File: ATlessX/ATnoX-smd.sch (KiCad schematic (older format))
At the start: 32 parts, among them J1 EXT_PWR_SW, J2 ATX, J3 AT, J4 PWR_LED, SW1 Power, U1 74LS74, U2 74LS14, U3 L7905

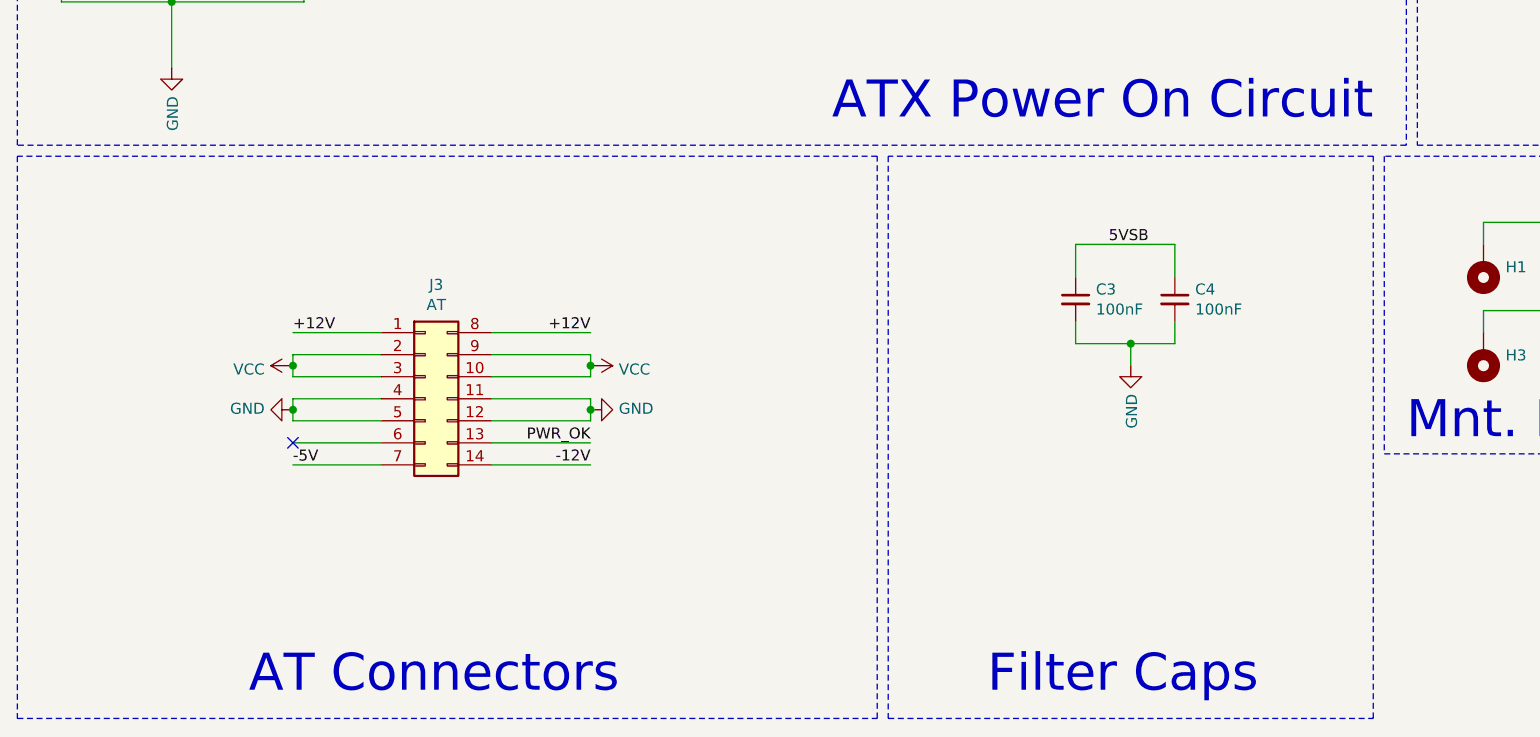
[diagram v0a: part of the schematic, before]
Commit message: Rev 3
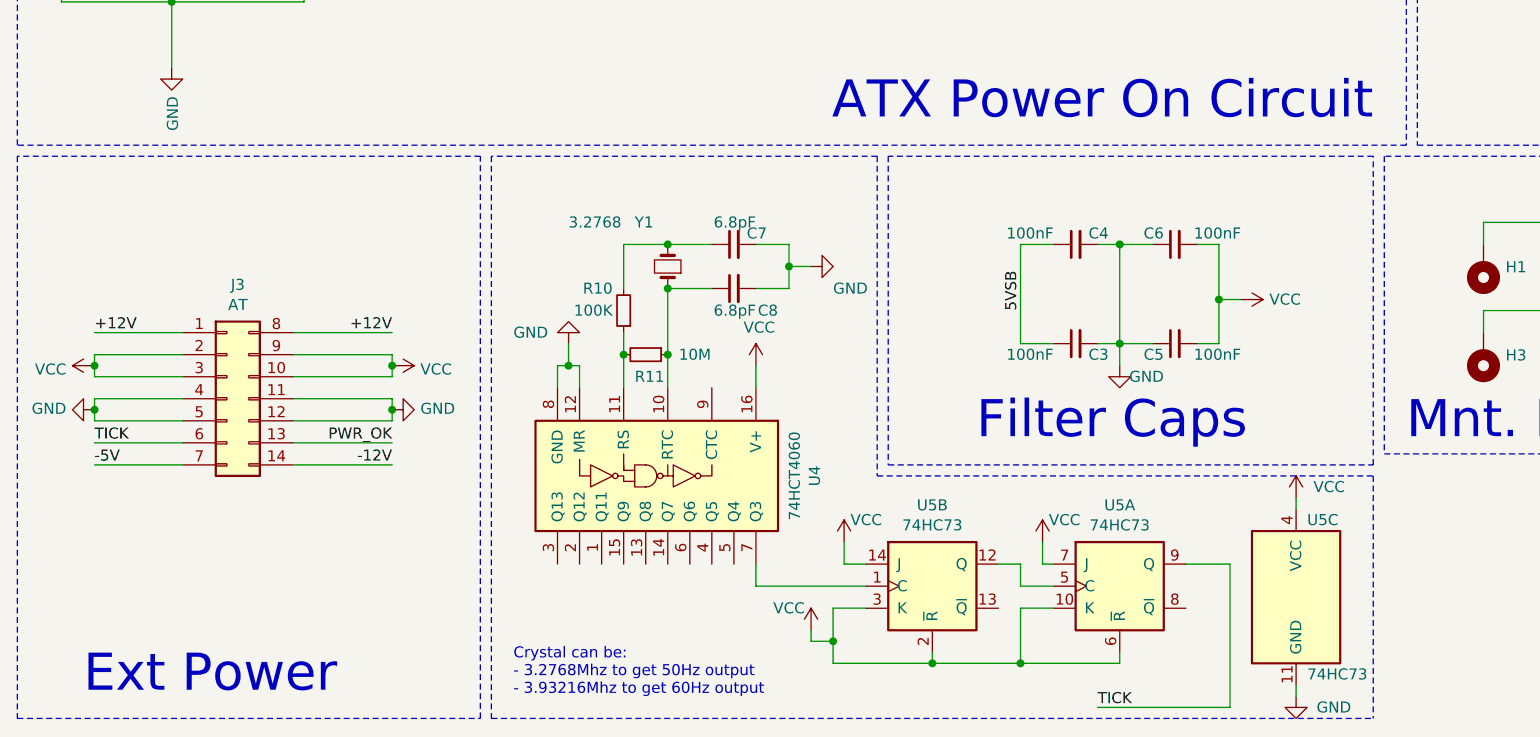
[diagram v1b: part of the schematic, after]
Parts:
- added C5, C6: 100nF, Capacitor_SMD:C_1206_3216Metric_Pad1.42x1.75mm_HandSolder, symbol Device:C_Small
- added C7, C8: 6.8pF, Capacitor_SMD:C_1206_3216Metric_Pad1.42x1.75mm_HandSolder, symbol Device:C_Small
- added R10: 100K, Resistor_SMD:R_1206_3216Metric_Pad1.42x1.75mm_HandSolder, symbol Device:R_Small
- added R11: 10M, Resistor_SMD:R_1206_3216Metric_Pad1.42x1.75mm_HandSolder, symbol Device:R_Small
- added U4: 74HCT4060, Package_SO:SOIC-16_3.9x9.9mm_P1.27mm, symbol logic-4000:4060-SO
- added U5: 74HC73, Package_SO:SOIC-14_3.9x8.7mm_P1.27mm, symbol 74xx:74LS73
- added Y1: 3.2768, Crystal:Crystal_SMD_HC49-SD, symbol Device:Crystal_Small
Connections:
- net GND: now also C5.1, C6.1, C7.2, C8.2, U4.12 (MR), U4.8 (GND), U5.11 (GND)
- net VCC: now also C5.2, C6.2, U4.16 (V+), U5.10 (K), U5.14 (J), U5.2 (~R), U5.3 (K), U5.4 (VCC), U5.6 (~R), U5.7 (J)
- net TICK: now reaches J3.6 (Pin_6)
- net TICK: now also U5.9 (Q)
- new net: C8.1, R11.1, U4.10 (RTC), Y1.1
- new net: R10.1, R11.2, U4.11 (RS)
- new net: U4.7 (Q3), U5.1 (C)
- new net: C7.1, R10.2, Y1.2
- new net: U5.12 (Q), U5.5 (C)
- no-connect marks 12 -> 11
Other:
- note added: "Crystal can be:\n- 3.2768Mhz to get 50Hz output\n- 3.93216Mhz to get 60Hz output"
- note added: "Ext Power"
- note removed: "AT Connectors"
- moved on the sheet: C3, C4, J3
